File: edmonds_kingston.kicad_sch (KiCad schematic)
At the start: 16 parts

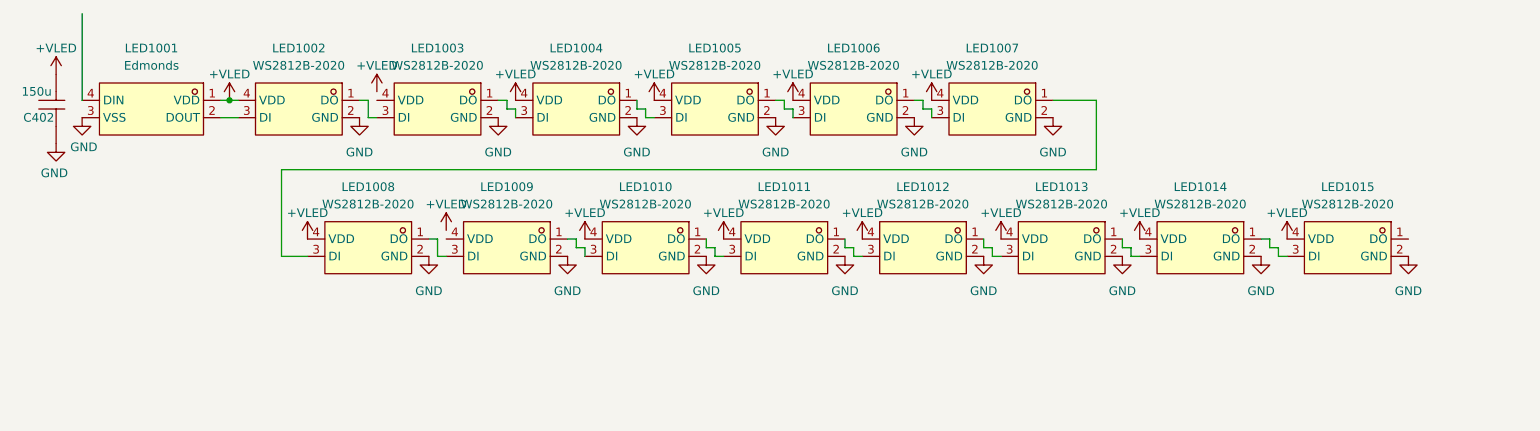
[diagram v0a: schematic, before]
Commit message: routing complete
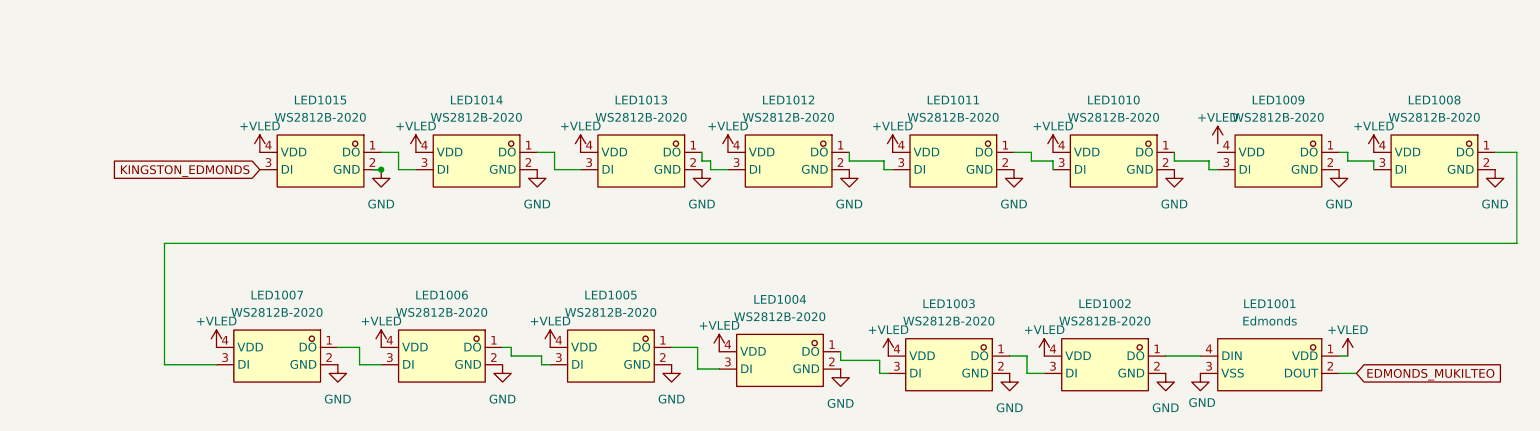
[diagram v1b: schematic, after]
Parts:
- removed C402: 150u, EasyEDA:CAP-SMD_L3.5-W2.8, symbol EasyEDA:CL21B106KOQNNNE
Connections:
- net +VLED: now also LED1003.4 (VDD)
- net at LED1004.1 (DO): now also LED1003.3 (DI); no longer LED1005.3 (DI)
- net at LED1003.1 (DO): now also LED1002.3 (DI); no longer LED1004.3 (DI)
- net at LED1014.1 (DO): now also LED1013.3 (DI); no longer LED1015.3 (DI)
- net at LED1013.1 (DO): now also LED1012.3 (DI); no longer LED1014.3 (DI)
- net at LED1015.1 (DO): now also LED1014.3 (DI)
- net at LED1010.3 (DI): now also LED1011.1 (DO); no longer LED1009.1 (DO)
- net at LED1009.3 (DI): now also LED1010.1 (DO); no longer LED1008.1 (DO)
- net at LED1012.1 (DO): now also LED1011.3 (DI); no longer LED1013.3 (DI)
- net at LED1002.1 (DO): now also LED1001.4 (DIN); no longer LED1003.3 (DI)
- net EDMONDS_MUKILTEO: now reaches LED1001.2 (DOUT)
- net EDMONDS_MUKILTEO: no longer LED1002.3 (DI)
- net at LED1007.3 (DI): now also LED1008.1 (DO); no longer LED1006.1 (DO)
- net at LED1005.1 (DO): now also LED1004.3 (DI); no longer LED1006.3 (DI)
- net at LED1008.3 (DI): now also LED1009.1 (DO); no longer LED1007.1 (DO)
- new net: LED1005.3 (DI), LED1006.1 (DO)
- new net: LED1006.3 (DI), LED1007.1 (DO)
- new net KINGSTON_EDMONDS: LED1015.3 (DI)
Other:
- moved on the sheet: LED1001
